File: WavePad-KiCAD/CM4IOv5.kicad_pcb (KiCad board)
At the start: 4 copper layers, 56.5 x 67.9 mm, 21 parts, among them J15 Conn_01x22_Female, J5 USB_C_Receptacle_USB2.0_14P, J7 Micro_SD_Card_Det, J8 Conn_01x22_Female, U1 USBLC6-4SC6, U18 RT9742GGJ5, U5 74LVC1G07SE-7

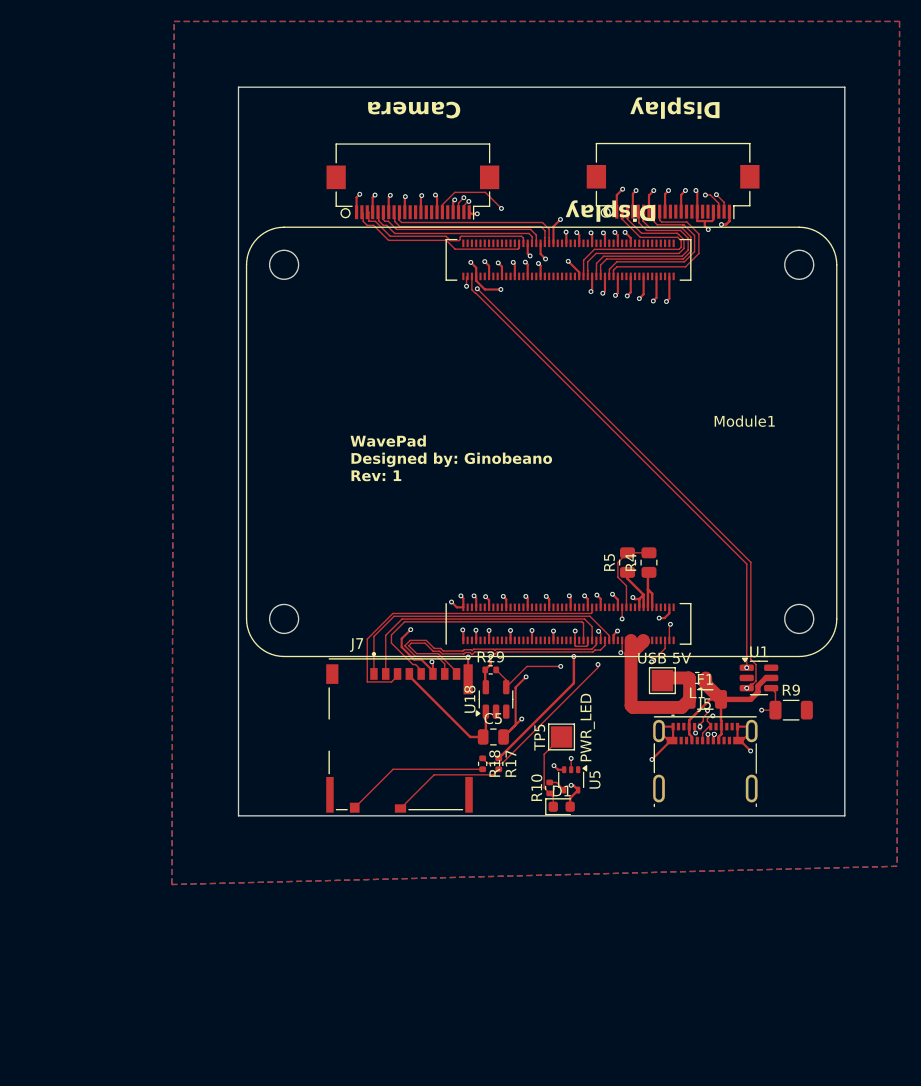
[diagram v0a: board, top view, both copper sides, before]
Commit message: Finish PCB Design
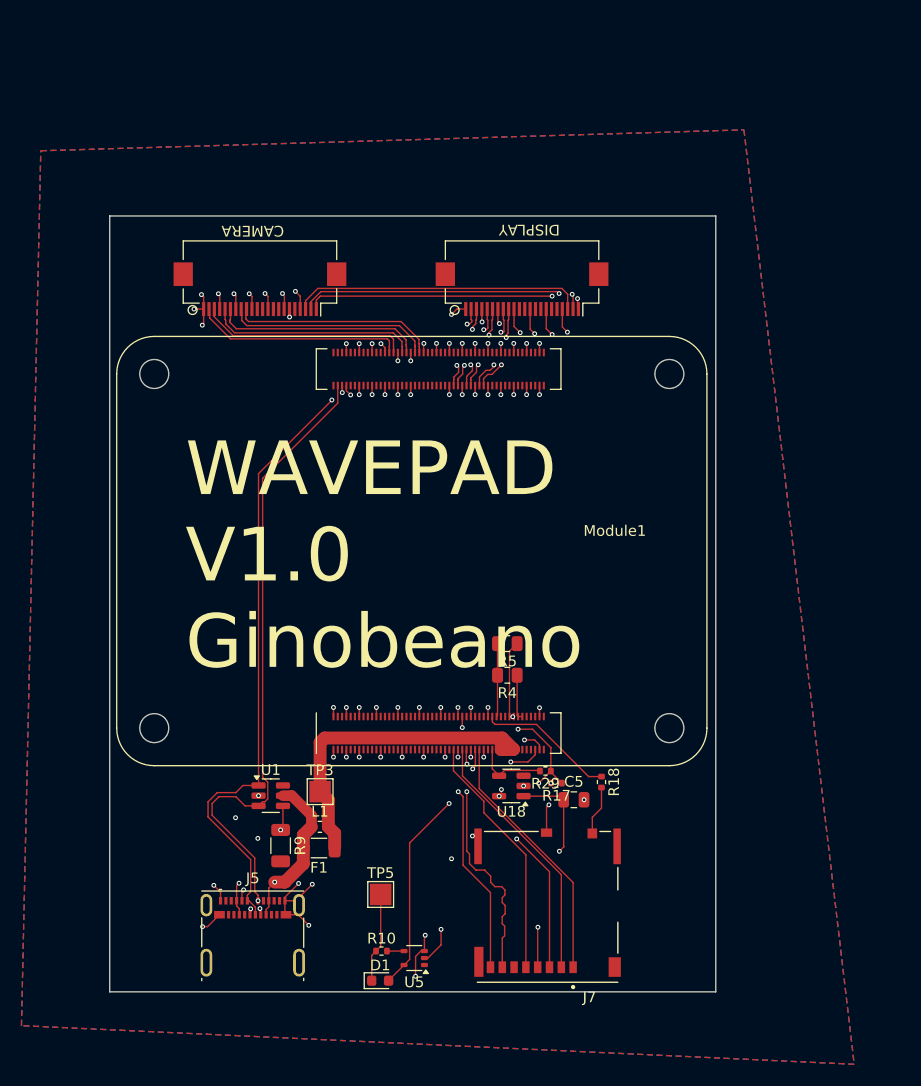
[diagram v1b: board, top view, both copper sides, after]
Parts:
- moved R9 49.2 mm to (122.4, 109.4), turned to -90 degrees
- moved U1 46.8 mm to (121.5, 104.7)
- moved J5 45.2 mm to (119.8, 117.7)
- moved F1 38.6 mm to (126.0, 109.6), turned to 180 degrees
- moved L1 37.8 mm to (126.1, 107.6), turned to 0 degrees
- moved TP3 33.5 mm to (126.1, 104.3)
- moved D1 23.4 mm to (131.7, 122.0)
- moved TP5 22.3 mm to (131.8, 113.9), turned to 0 degrees
- moved U5 22.1 mm to (134.9, 119.8), turned to 180 degrees
- moved R10 21.8 mm to (131.8, 119.2), turned to 0 degrees
- moved J7 21.2 mm to (147.3, 115.1), turned to 180 degrees
- moved J8 16.9 mm to (120.5, 57.5)
- moved R4 16.9 mm to (143.6, 93.5), turned to 180 degrees
- moved J15 16.7 mm to (144.9, 57.5)
- moved Module1 15.8 mm to (158.7, 98.4)
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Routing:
- net GND: track 125.3 -> 90.2 mm, vias 67 -> 81
- net /+5v: track 18.2 -> 30.2 mm
- net /CM4_HighSpeed/DSI0_D0_N: track 18.7 -> 8.19 mm, vias 0 -> 2
- net /CM4_HighSpeed/DSI0_D0_P: track 18.4 -> 8.43 mm, vias 0 -> 2
- net /CM4_GPIO (GPIO, SDCARD)/nPWR_LED: track 15.7 -> 24.8 mm
- net /CM4_HighSpeed/DSI0_D1_P: track 17.3 -> 8.27 mm, vias 0 -> 2
- net /CM4_HighSpeed/DSI0_D1_N: track 17.6 -> 8.59 mm, vias 0 -> 2
- net Net-(J7-DET_B): track 13.4 -> 4.63 mm
- net /CM4_GPIO (GPIO, SDCARD)/SD_PWR_ON: track 15.4 -> 6.73 mm, vias 2 -> 0
- net /CM4_GPIO (GPIO, SDCARD)/SD_PWR: track 11.9 -> 20.5 mm, vias 0 -> 2
- net /CM4_GPIO (GPIO, SDCARD)/Reserved: track 21.2 -> 12.8 mm, vias 2 -> 0
- net /+3.3v: track 54.0 -> 46.3 mm, vias 4 -> 6
- net /CM4_HighSpeed/DSI0_C_N: track 16.0 -> 8.53 mm, vias 0 -> 2
- net /CM4_HighSpeed/DSI0_C_P: track 16.0 -> 9.07 mm, vias 0 -> 2
- net Net-(J7-DET_A): track 10.7 -> 4.79 mm, vias 0 -> 2
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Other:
- board size 56.5 x 67.9 mm -> 56.5 x 72.3 mm
- board text added: "CAMERA"
- board text added: "DISPLAY"
- board text added: "WAVEPAD V1.0 Ginobeano"
- board text removed: "Camera"
- board text removed: "Display"
- board text removed: "PWR_LED"
- board text removed: "USB 5V"
- board text removed: "WavePad Designed by: Ginobeano Rev: 1"
